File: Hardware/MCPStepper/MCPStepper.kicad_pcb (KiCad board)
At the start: 2 copper layers, 48.3 x 78 mm, 22 parts, among them J1 Conn_01x05, J2 Conn_01x05, J3 Conn_01x05, J4 Conn_01x05, J5 Conn_01x02, J6 Conn_01x05, J7 Conn_01x03, J8 Conn_01x03, J9 Conn_01x03, U1 MCP23017_SP, U2 ULN2003A, U3 ULN2003A, U4 ULN2003A

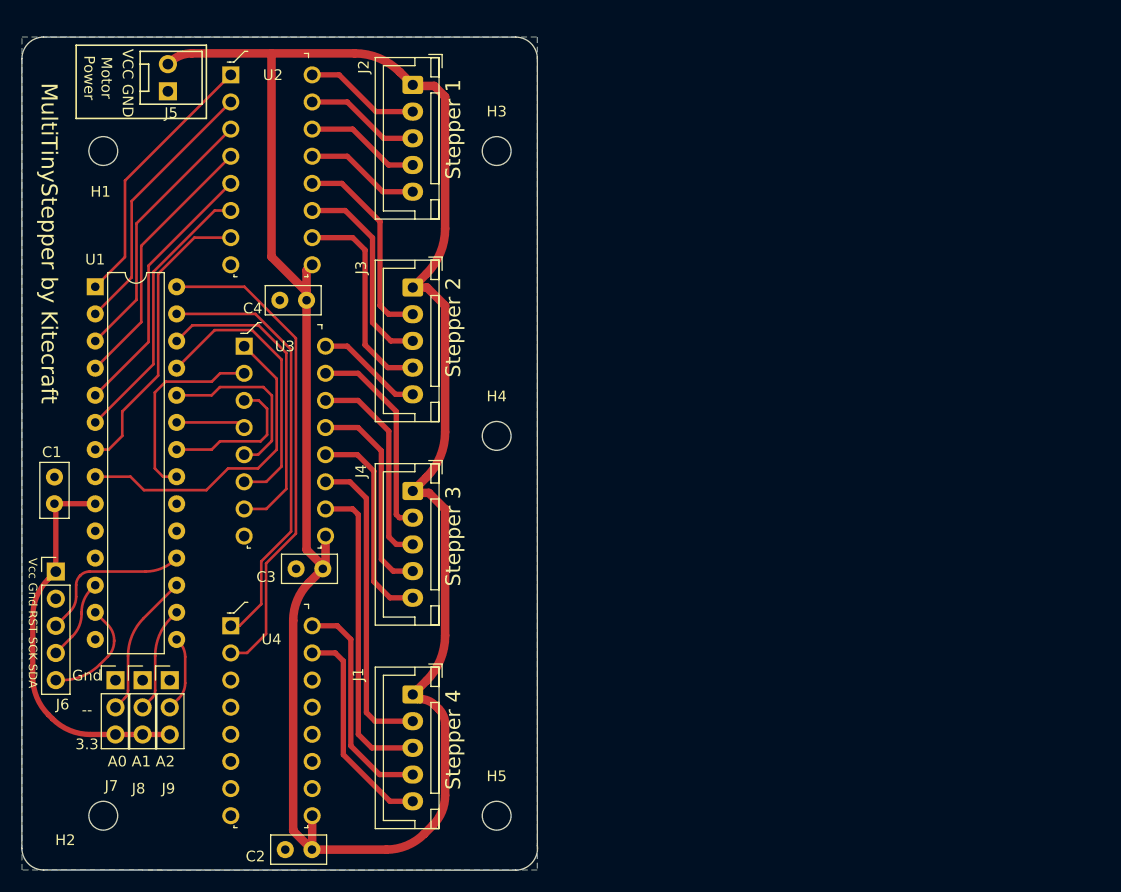
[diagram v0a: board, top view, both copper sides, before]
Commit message: PCB Updates
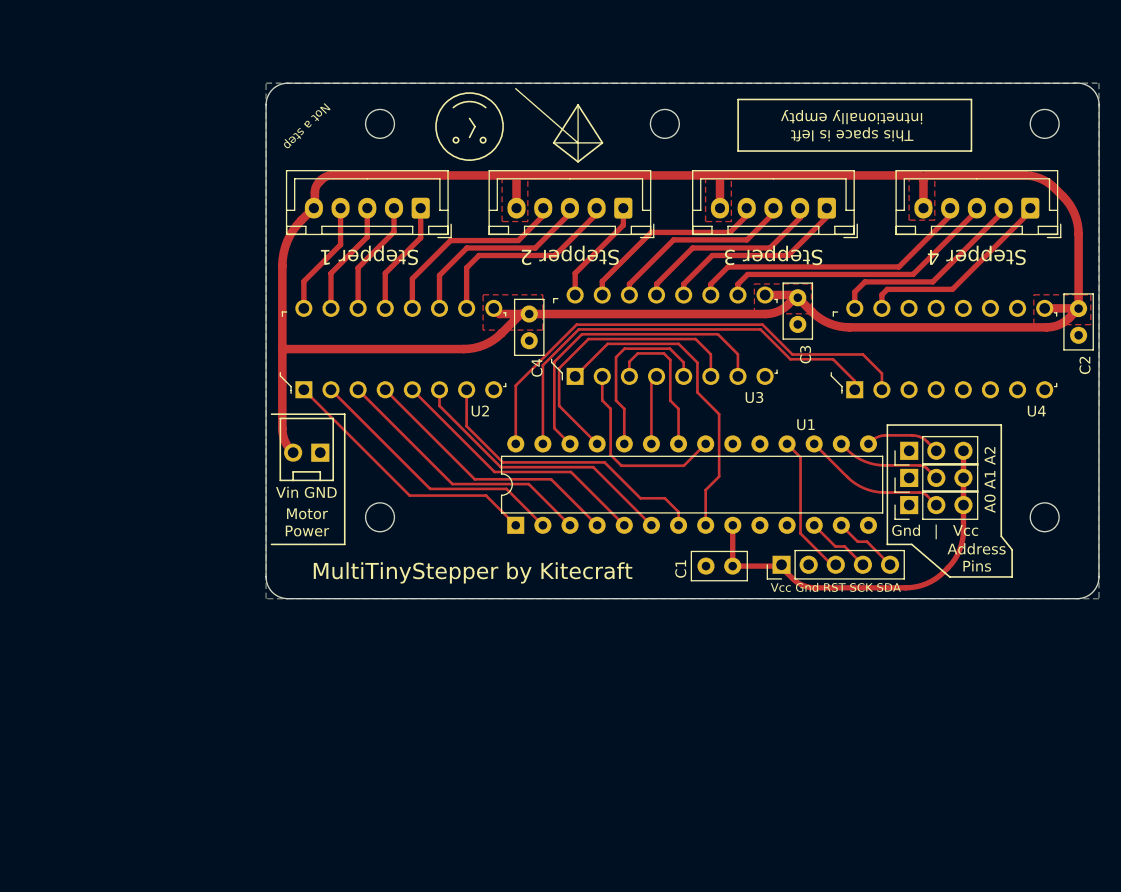
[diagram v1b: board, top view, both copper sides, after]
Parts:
- moved H2 92.5 mm to (166.9, 113.0), turned to 90 degrees
- moved C2 88.5 mm to (170.1, 96.0), turned to 90 degrees
- moved H5 82.6 mm to (166.9, 76.2), turned to 90 degrees
- moved J7 76.1 mm to (154.2, 111.9), turned to 90 degrees
- moved J8 74.2 mm to (154.2, 109.3), turned to 90 degrees
- moved J1 73.6 mm to (165.5, 84.1), turned to 180 degrees
- moved J9 72.5 mm to (154.2, 106.8), turned to 90 degrees
- moved J6 67.9 mm to (142.2, 117.5), turned to 90 degrees
- moved U4 62.5 mm to (149.1, 101.1), turned to 90 degrees
- moved C1 61.6 mm to (135.2, 117.6), turned to 0 degrees
- moved C3 52.2 mm to (143.8, 95.0), turned to 90 degrees
- moved J4 46.9 mm to (146.5, 84.1), turned to 180 degrees
- moved U1 45.3 mm to (117.4, 113.8), turned to 90 degrees
- moved H1 43.0 mm to (104.6, 113.0), turned to 90 degrees
- moved J5 38.2 mm to (96.5, 107.0), turned to -90 degrees
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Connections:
- J1 pad 1: VCC -> Net-(U4-Pad15)
- J1 pad 2: Net-(J1-Pad2) -> Net-(U4-Pad16)
- J1 pad 4: Net-(J1-Pad4) -> Net-(U3-Pad11)
- J1 pad 5: Net-(J1-Pad5) -> VCC
- J2 pad 1: VCC -> Net-(U2-Pad13)
- J2 pad 2: Net-(J2-Pad2) -> Net-(U2-Pad14)
- J2 pad 4: Net-(J2-Pad4) -> Net-(U2-Pad16)
- J2 pad 5: Net-(J2-Pad5) -> VCC
- J3 pad 1: VCC -> Net-(J3-Pad1)
- J3 pad 5: Net-(J3-Pad5) -> VCC
- J4 pad 1: VCC -> Net-(U3-Pad12)
- J4 pad 2: Net-(J4-Pad2) -> Net-(U3-Pad13)
- J4 pad 4: Net-(J4-Pad4) -> Net-(U3-Pad15)
- J4 pad 5: Net-(J4-Pad5) -> VCC
- U2 pad 10: Net-(J3-Pad4) -> Net-(J3-Pad2)
- U2 pad 12: Net-(J3-Pad2) -> Net-(J3-Pad4)
- U2 pad 13: Net-(J2-Pad5) -> Net-(U2-Pad13)
- U2 pad 14: Net-(J2-Pad4) -> Net-(U2-Pad14)
- U2 pad 16: Net-(J2-Pad2) -> Net-(U2-Pad16)
- U3 pad 11: Net-(J1-Pad2) -> Net-(U3-Pad11)
- U3 pad 12: Net-(J4-Pad5) -> Net-(U3-Pad12)
- U3 pad 13: Net-(J4-Pad4) -> Net-(U3-Pad13)
- U3 pad 15: Net-(J4-Pad2) -> Net-(U3-Pad15)
- U3 pad 16: Net-(J3-Pad5) -> Net-(J3-Pad1)
- U4 pad 15: Net-(J1-Pad5) -> Net-(U4-Pad15)
- U4 pad 16: Net-(J1-Pad4) -> Net-(U4-Pad16)
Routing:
- net Net-(J1-Pad2): track 29.2 -> 0.00 mm
- net Net-(U3-Pad11): track 0.00 -> 26.8 mm
- net Net-(J1-Pad4): track 21.0 -> 0.00 mm
- net Net-(J1-Pad5): track 20.3 -> 0.00 mm
- net Net-(J4-Pad5): track 19.8 -> 0.00 mm
- net Net-(J4-Pad4): track 19.7 -> 0.00 mm
- net Net-(J4-Pad2): track 19.4 -> 0.00 mm
- net Net-(U4-Pad16): track 0.00 -> 18.9 mm
- net Net-(U4-Pad15): track 0.00 -> 18.7 mm
- net Net-(U3-Pad15): track 0.00 -> 18.1 mm
- net Net-(U3-Pad13): track 0.00 -> 18.0 mm
- net Net-(U3-Pad12): track 0.00 -> 17.9 mm
- net Net-(U2-Pad16): track 0.00 -> 10.8 mm
- net Net-(J2-Pad2): track 10.8 -> 0.00 mm
- net Net-(J2-Pad4): track 10.8 -> 0.00 mm
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- added copper zone on F.Cu, net VCC
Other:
- board size 48.3 x 78 mm -> 78 x 48.3 mm
- board text added: "Address Pins"
- board text added: "Gnd"
- board text added: "Not a step"
- board text added: "This space is left intnetionally empty"
- board text added: "Vcc"
- board text added: "Vin GND"
- board text added: "|"
- board text removed: "Gnd -- 3.3"
- board text removed: "VCC GND"
